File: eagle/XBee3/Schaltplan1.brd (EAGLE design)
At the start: 102.8 x 84.8 mm, 61 parts, among them IC1 XB3-24Z8CM-J, IC2 317EMP, U1 CONNECTOR_6PIN, X1 22-23-2021, X2 22-23-2031, X3 22-23-2021

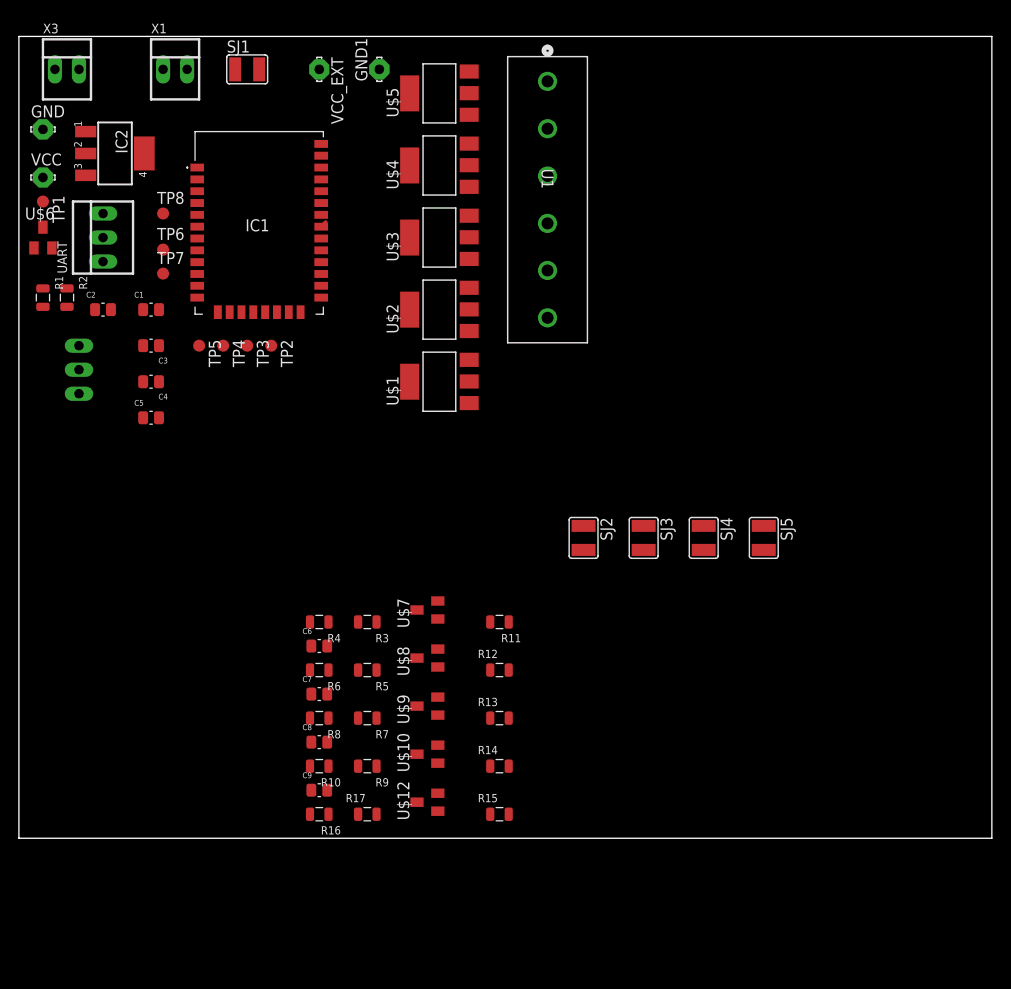
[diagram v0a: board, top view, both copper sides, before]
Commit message: Board rev0.2
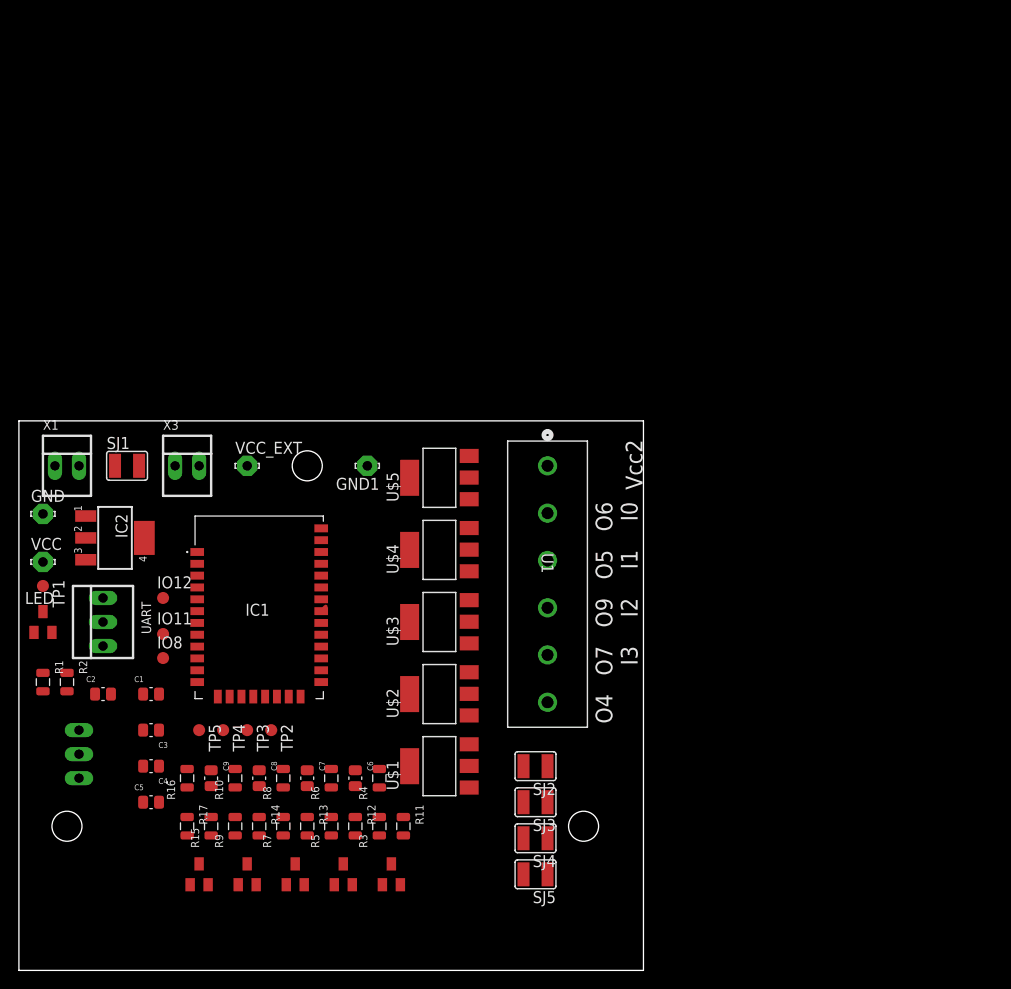
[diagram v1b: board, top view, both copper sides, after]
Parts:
- removed TP6, TP7, TP8: TPSQB1,27, testpad:B1,27
- removed U$6: LED_RG_SOT23, ROT_GRÜN_LED_SOT23:SOT23
- added IO11, IO12, IO8: TPSQB1,27, testpad:B1,27
- added LED: LED_RG_SOT23, ROT_GRÜN_LED_SOT23:SOT23
- moved SJ1 43.8 mm to (11.4, 54.6)
- moved X3 43.8 mm to (17.8, 54.6)
- moved X1 43.4 mm to (5.08, 54.6)
- moved SJ5 43.0 mm to (54.6, 11.4), turned to 180 degrees
- moved VCC_EXT 42.6 mm to (24.1, 54.6), turned to 0 degrees
- moved GND1 41.9 mm to (36.8, 54.6), turned to 180 degrees
- moved C1 40.6 mm to (14.0, 30.5)
- moved C2 40.6 mm to (8.89, 30.5)
- moved C3 40.6 mm to (14.0, 26.7)
- moved C4 40.6 mm to (14.0, 22.9)
- moved C5 40.6 mm to (14.0, 19.1)
- moved GND 40.6 mm to (2.54, 49.5)
- moved IC1 40.6 mm to (25.4, 31.8)
- moved R1 40.6 mm to (2.54, 31.8)
- moved R2 40.6 mm to (5.08, 31.8)
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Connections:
- net N$10: now also U1.3; no longer U1.2
- net N$11: now also U1.4; no longer U1.3
- net N$12: now also U1.5; no longer U1.4
- net N$13: now also U1.6; no longer U1.5
- net N$14: now also U1.1; no longer U1.6
- net N$25: now also LED.1; no longer U$6.1
- net N$26: now also LED.2; no longer U$6.2
- net N$3: now also IO12.TP; no longer TP8.TP
- net N$34: now also IO11.TP; no longer TP6.TP
- net N$35: now also IO8.TP; no longer TP7.TP
- net N$43: now also LED.3; no longer U$6.3
- net N$9: now also U1.2; no longer U1.1
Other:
- board size 102.8 x 84.8 mm -> 66 x 58.1 mm
- board text added: "O4"
- board text added: "O5 I1"
- board text added: "O6 I0"
- board text added: "O7 I3"
- board text added: "O9 I2"
- board text added: "Vcc2"
